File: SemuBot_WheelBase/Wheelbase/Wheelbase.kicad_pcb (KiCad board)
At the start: 2 copper layers, 60 x 60 mm, 71 parts, among them IC1 NCP164CSN330T1G, J1 10155435-00011LF, J2 ftsh-105-01-l-dv-k, J3 TB003-500-P02BE, J4 B5B-XH-A_LF__SN_, J5 B5B-XH-A_LF__SN_, J6 B5B-XH-A_LF__SN_, J7 1984620, J8 1984620, J9 1984620, Q1 DI025N06PT-AQ, Q10 DI025N06PT-AQ, Q11 DI025N06PT-AQ, Q12 DI025N06PT-AQ, Q13 DI025N06PT-AQ, Q14 DI025N06PT-AQ, Q15 DI025N06PT-AQ, Q16 DI025N06PT-AQ, Q17 DI025N06PT-AQ, Q18 DI025N06PT-AQ, Q2 DI025N06PT-AQ, Q3 DI025N06PT-AQ, Q4 DI025N06PT-AQ, Q5 DI025N06PT-AQ, Q6 DI025N06PT-AQ, Q7 DI025N06PT-AQ, Q8 DI025N06PT-AQ, Q9 DI025N06PT-AQ, U1 STM32F303RET6, U2 DRV8353FSRTAR, U3 DRV8353FSRTAR, U4 DRV8353FSRTAR, Y1 WE-SPXO_CFPS-39

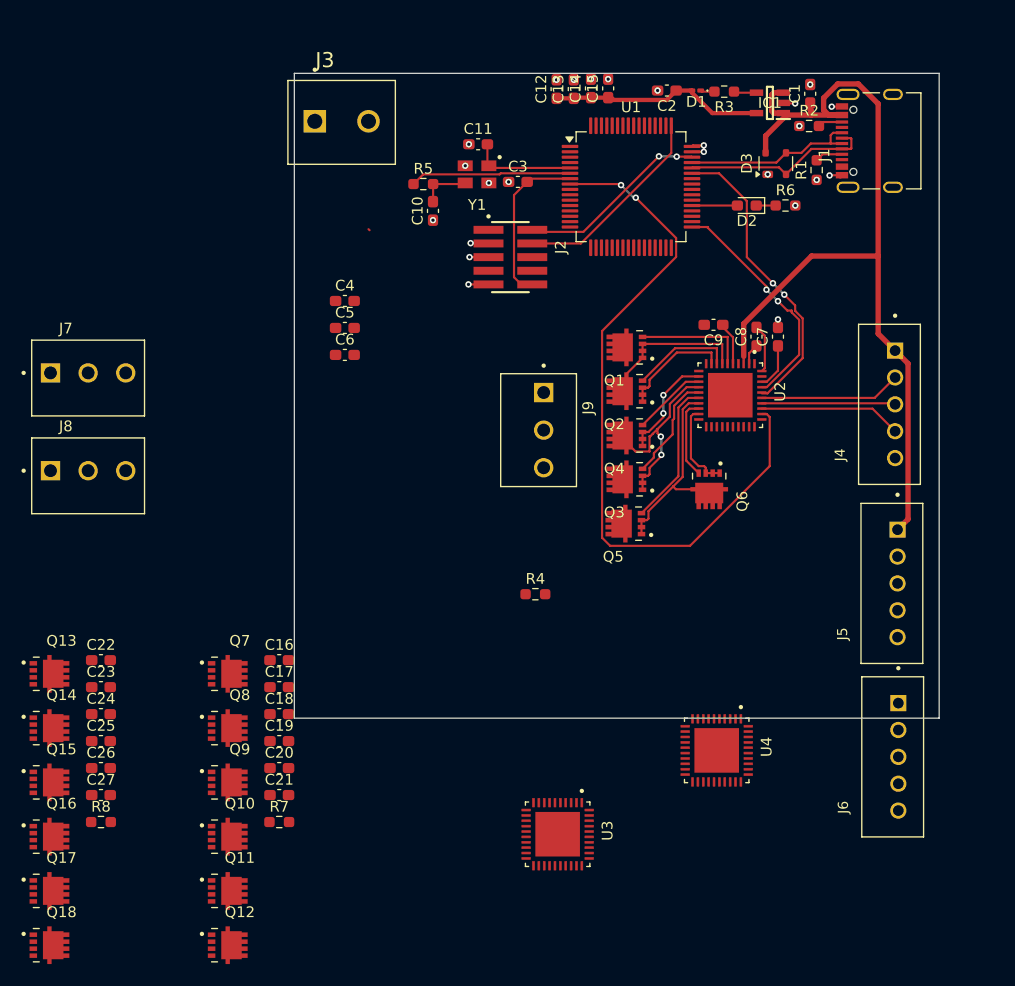
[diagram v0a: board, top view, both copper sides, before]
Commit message: Snapshot
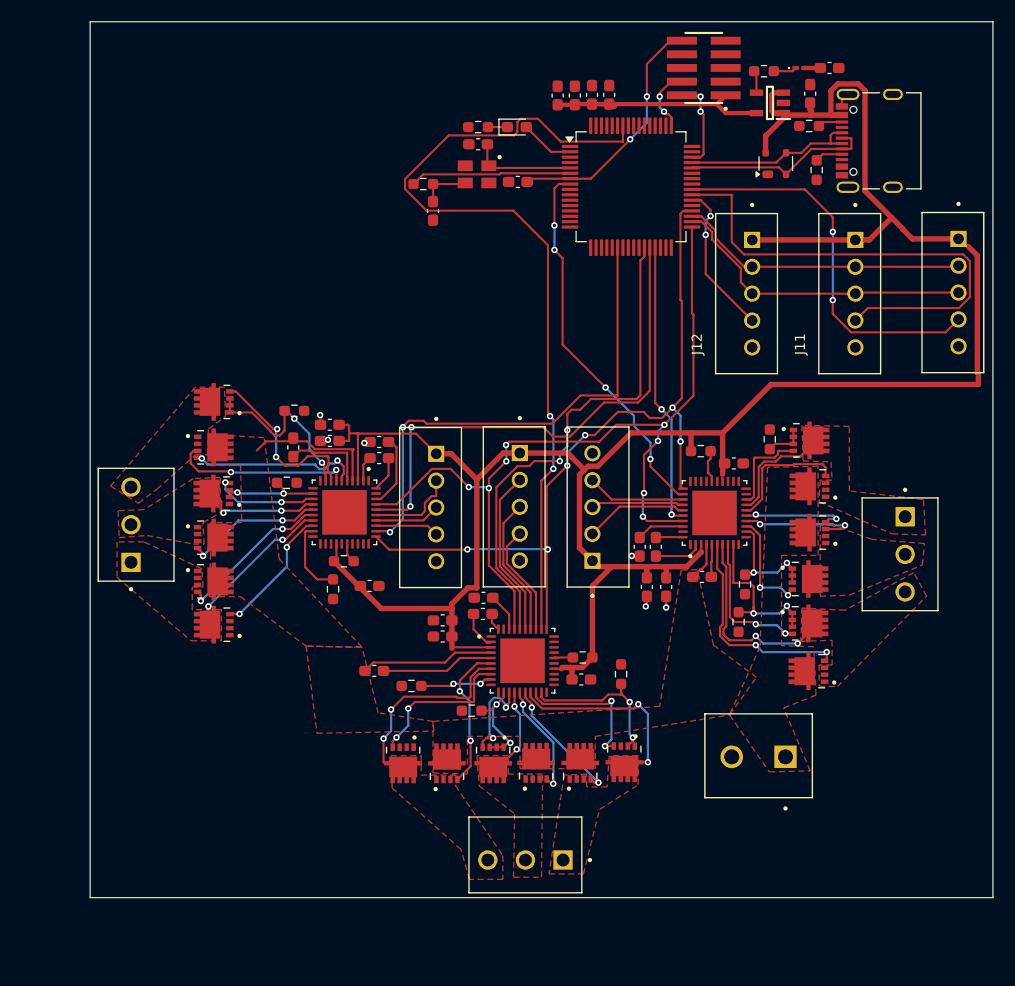
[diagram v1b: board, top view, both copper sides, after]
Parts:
- added J10: B5B-XH-A_LF__SN_, B5B-XH-A_LF__SN_:JST_B5B-XH-A_LF__SN_, F.Cu at (192.9, 74.5)
- added J11: B5B-XH-A_LF__SN_, B5B-XH-A_LF__SN_:JST_B5B-XH-A_LF__SN_, F.Cu at (183.3, 74.5)
- added J12: B5B-XH-A_LF__SN_, B5B-XH-A_LF__SN_:JST_B5B-XH-A_LF__SN_, F.Cu at (173.8, 74.5)
- added R10: 1k, Resistor_SMD:R_0603_1608Metric_Pad0.98x0.95mm_HandSolder, F.Cu at (131.7, 85.5)
- added R11: 1k, Resistor_SMD:R_0603_1608Metric_Pad0.98x0.95mm_HandSolder, F.Cu at (142.6, 111.0)
- added R12: 1k, Resistor_SMD:R_0603_1608Metric_Pad0.98x0.95mm_HandSolder, F.Cu at (175.9, 88.1)
- added R13: 1k, Resistor_SMD:R_0603_1608Metric_Pad0.98x0.95mm_HandSolder, F.Cu at (135.3, 102.0)
- added R14: 1k, Resistor_SMD:R_0603_1608Metric_Pad0.98x0.95mm_HandSolder, F.Cu at (162.1, 110.0)
- added R15: 1k, Resistor_SMD:R_0603_1608Metric_Pad0.98x0.95mm_HandSolder, F.Cu at (173.6, 101.6)
- added R16: 1k, Resistor_SMD:R_0603_1608Metric_Pad0.98x0.95mm_HandSolder, F.Cu at (131.0, 92.2)
- added R17: 1k, Resistor_SMD:R_0603_1608Metric_Pad0.98x0.95mm_HandSolder, F.Cu at (148.2, 113.3)
- added R9: 1k, Resistor_SMD:R_0603_1608Metric_Pad0.98x0.95mm_HandSolder, F.Cu at (173.0, 105.1)
- moved J3 73.6 mm to (177.4, 117.7), turned to 180 degrees
- moved J7 63.4 mm to (158.4, 123.2), turned to 180 degrees
- moved Q18 56.1 mm to (162.4, 118.2), turned to -90 degrees
- moved Q17 50.8 mm to (158.3, 118.2), turned to 90 degrees
- moved R8 47.4 mm to (158.5, 108.4)
- moved Q15 45.3 mm to (154.2, 118.2), turned to 90 degrees
- moved C24 44.8 mm to (158.4, 110.5)
- moved J5 43.5 mm to (144.3, 94.5)
- moved J6 42.2 mm to (152.1, 94.4)
- moved Q16 41.9 mm to (150.2, 118.2), turned to -90 degrees
- moved C4 38.7 mm to (164.5, 101.8), turned to -90 degrees
- moved C5 38.4 mm to (166.3, 101.8), turned to -90 degrees
- moved C26 38.3 mm to (149.2, 104.3)
- moved C25 38.0 mm to (149.3, 102.8), turned to 180 degrees
- moved Q13 37.9 mm to (145.9, 118.2), turned to 90 degrees
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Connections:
- J3 pad 1: PGND -> +24V
- J3 pad 2: +24V -> PGND
- J7 pad 1: /Motor_3/SHA -> /Motor_3/SHC
- J7 pad 3: /Motor_3/SHC -> /Motor_3/SHA
- J8 pad 1: /Motor_2/SHA -> /Motor_2/SHC
- J8 pad 3: /Motor_2/SHC -> /Motor_2/SHA
- J9 pad 1: /Motor_1/SHA -> /Motor_1/SHC
- J9 pad 3: /Motor_1/SHC -> /Motor_1/SHA
- U1 pad 2: unconnected-(U1-PC13-Pad2) -> Net-(D2-A)
- U1 pad 27: unconnected-(U1-PB1-Pad27) -> /MOTOR3_DIR
- U1 pad 28: unconnected-(U1-PB2-Pad28) -> /MOTOR2_DIR
- U1 pad 29: unconnected-(U1-PB10-Pad29) -> /MOTOR1_DIR
- U1 pad 34: unconnected-(U1-PB13-Pad34) -> /SPI_CLK
- U1 pad 35: unconnected-(U1-PB14-Pad35) -> /SPI_DATA
- U1 pad 37: Net-(D2-A) -> unconnected-(U1-PC6-Pad37)
- U1 pad 41: /MOTOR3_DIR -> unconnected-(U1-PA8-Pad41)
- U1 pad 42: /MOTOR2_DIR -> unconnected-(U1-PA9-Pad42)
- U1 pad 43: /MOTOR1_DIR -> unconnected-(U1-PA10-Pad43)
- U2 pad 10: unconnected-(U2-SNA-Pad10) -> PGND
- U2 pad 11: unconnected-(U2-SNB-Pad11) -> PGND
- U2 pad 20: unconnected-(U2-SNC-Pad20) -> PGND
- U3 pad 10: unconnected-(U3-SNA-Pad10) -> PGND
- U3 pad 11: unconnected-(U3-SNB-Pad11) -> PGND
- U3 pad 20: unconnected-(U3-SNC-Pad20) -> PGND
- U4 pad 10: unconnected-(U4-SNA-Pad10) -> PGND
- U4 pad 11: unconnected-(U4-SNB-Pad11) -> PGND
- U4 pad 20: unconnected-(U4-SNC-Pad20) -> PGND
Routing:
- net +5V: track 83.3 -> 218.7 mm
- net /MOTOR3_PWM: track 0.00 -> 78.3 mm, vias 0 -> 2
- net /ENABLE: track 0.00 -> 73.3 mm, vias 0 -> 6
- net /nBRAKE: track 21.9 -> 79.8 mm, vias 2 -> 8
- net /MOTOR2_DIR: track 0.00 -> 48.4 mm, vias 0 -> 2
- net /MOTOR3_DIR: track 0.00 -> 47.1 mm, vias 0 -> 2
- net /MOTOR2_PWM: track 0.00 -> 46.8 mm, vias 0 -> 2
- net /CS_ENC_2: track 0.00 -> 45.9 mm
- net /CS_ENC_1: track 0.00 -> 36.1 mm, vias 0 -> 2
- net /MOTOR1_PWM: track 67.1 -> 35.3 mm, vias 2 -> 4
- net /SPI_CLK: track 0.00 -> 28.8 mm
- net +24V: track 0.14 -> 28.7 mm
- net /SPI_DATA: track 0.00 -> 27.2 mm
- net /Motor_3/SHA: track 0.00 -> 19.1 mm, vias 0 -> 2
- net /Motor_3/SHC: track 0.00 -> 19.0 mm, vias 0 -> 2
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- added copper zone on F.Cu, net +24V
- added copper zone on F.Cu, net /Motor_1/SHA
- added copper zone on F.Cu, net /Motor_1/SHB
- added copper zone on F.Cu, net /Motor_1/SHC
- added copper zone on F.Cu, net /Motor_2/SHA
- added copper zone on F.Cu, net /Motor_2/SHB
- added copper zone on F.Cu, net /Motor_2/SHC
- added copper zone on F.Cu, net /Motor_3/SHA
- added copper zone on F.Cu, net /Motor_3/SHB
- added copper zone on F.Cu, net /Motor_3/SHC
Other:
- board size 60 x 60 mm -> 84 x 81.5 mm
- rule pad_to_mask_clearance: 0 -> 0.05
